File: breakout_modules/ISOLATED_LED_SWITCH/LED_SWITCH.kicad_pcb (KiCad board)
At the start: 2 copper layers, 26 x 24.8 mm, 13 parts, among them J1 TB001-500-02BE, J2 TB003V-500-P02BE, J3 SM04B-GHS-TB(LF)(SN), J4 01x07 2.54mm Pin headers, U1 TLP2710(TP4,E, U2 SI3402-TP

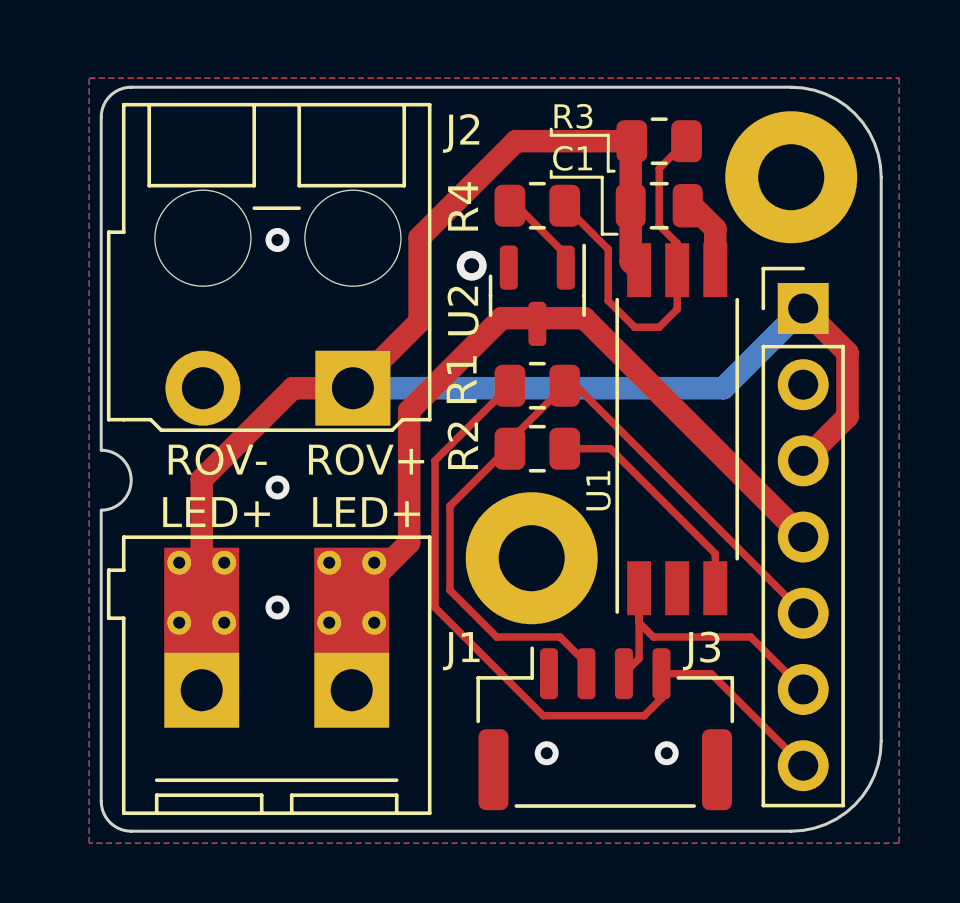
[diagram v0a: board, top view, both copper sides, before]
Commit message: Updated isolated PWM and isolated LED with barrel jack, fixed 2x2 to JST adapter board
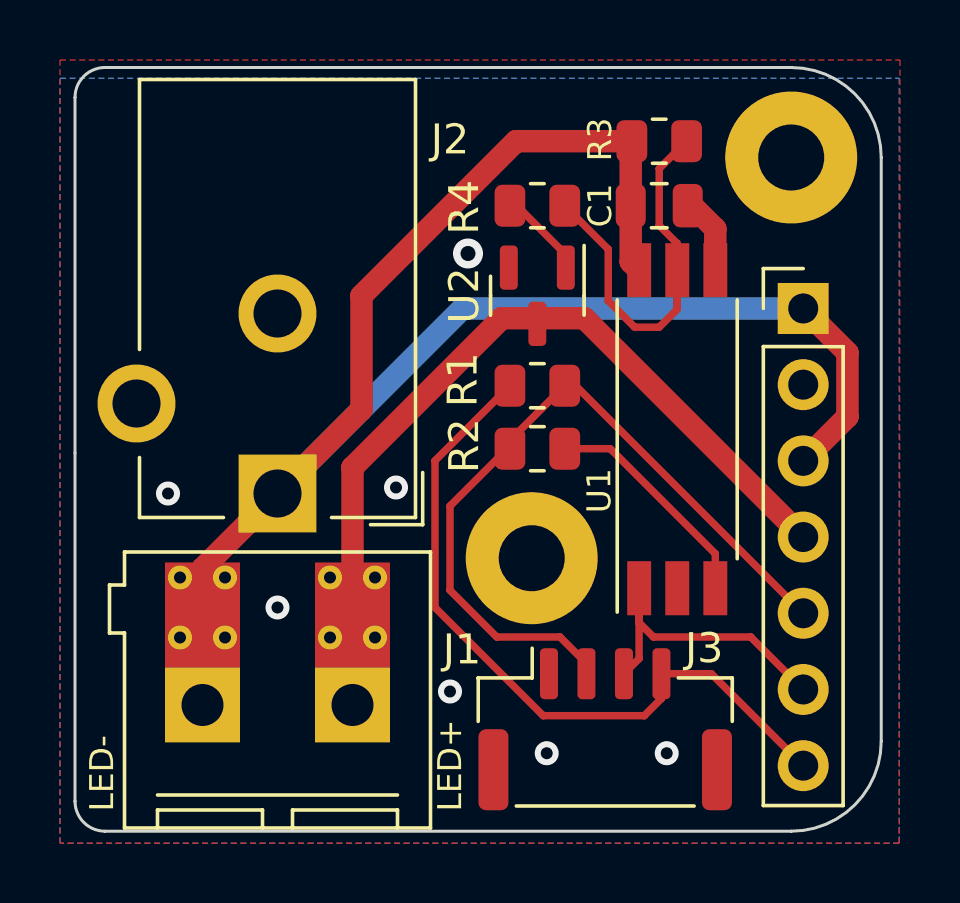
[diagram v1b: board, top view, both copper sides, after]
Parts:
- J2: value TB003V-500-P02BE -> Barrel_Jack; footprint 0_lib_fp:TB003V-500-P02BE -> Connector_BarrelJack:BarrelJack_CUI_PJ-102AH_Horizontal
- moved J2 3.51 mm to (140.2, 100.2)
- moved H2 0.66 mm to (157.4, 89.0)
- moved J1 0.49 mm to (140.2, 107.2)
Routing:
- net LED_ANODE+: track 51.5 -> 54.8 mm
- net GND: vias 6 -> 7
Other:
- board size 26 x 24.8 mm -> 26.9 x 25.5 mm
- board text removed: "ROV+"
- board text removed: "ROV-"

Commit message: Replaced barrel jacks with terminal blocks
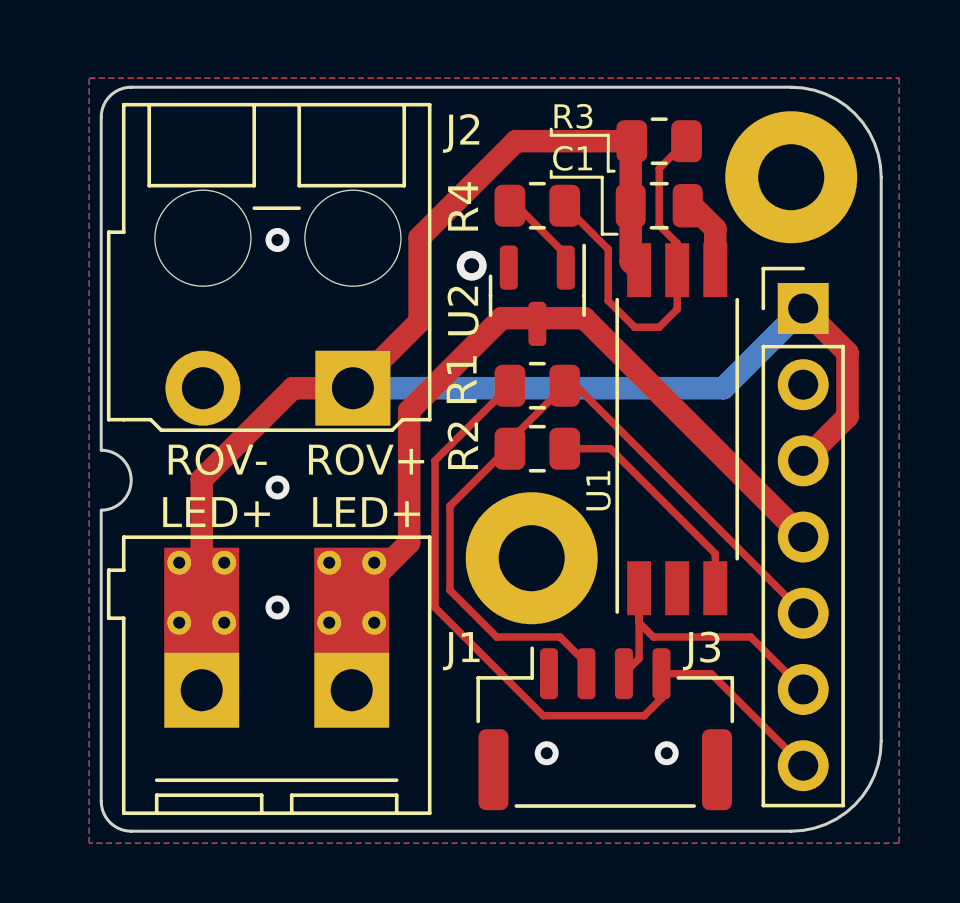
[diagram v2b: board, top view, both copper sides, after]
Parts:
- J2: value Barrel_Jack -> TB003V-500-P02BE; footprint Connector_BarrelJack:BarrelJack_CUI_PJ-102AH_Horizontal -> 0_lib_fp:TB003V-500-P02BE
- moved J2 3.51 mm to (140.2, 96.7)
- moved H2 0.66 mm to (157.4, 89.7)
- moved J1 0.49 mm to (140.2, 106.8)
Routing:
- net LED_ANODE+: track 54.8 -> 51.5 mm
- net GND: vias 7 -> 6
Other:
- board size 26.9 x 25.5 mm -> 26 x 24.8 mm
- board text added: "ROV+"
- board text added: "ROV-"
